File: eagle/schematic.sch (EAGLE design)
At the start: 4 parts, among them U1 SN74HC595N

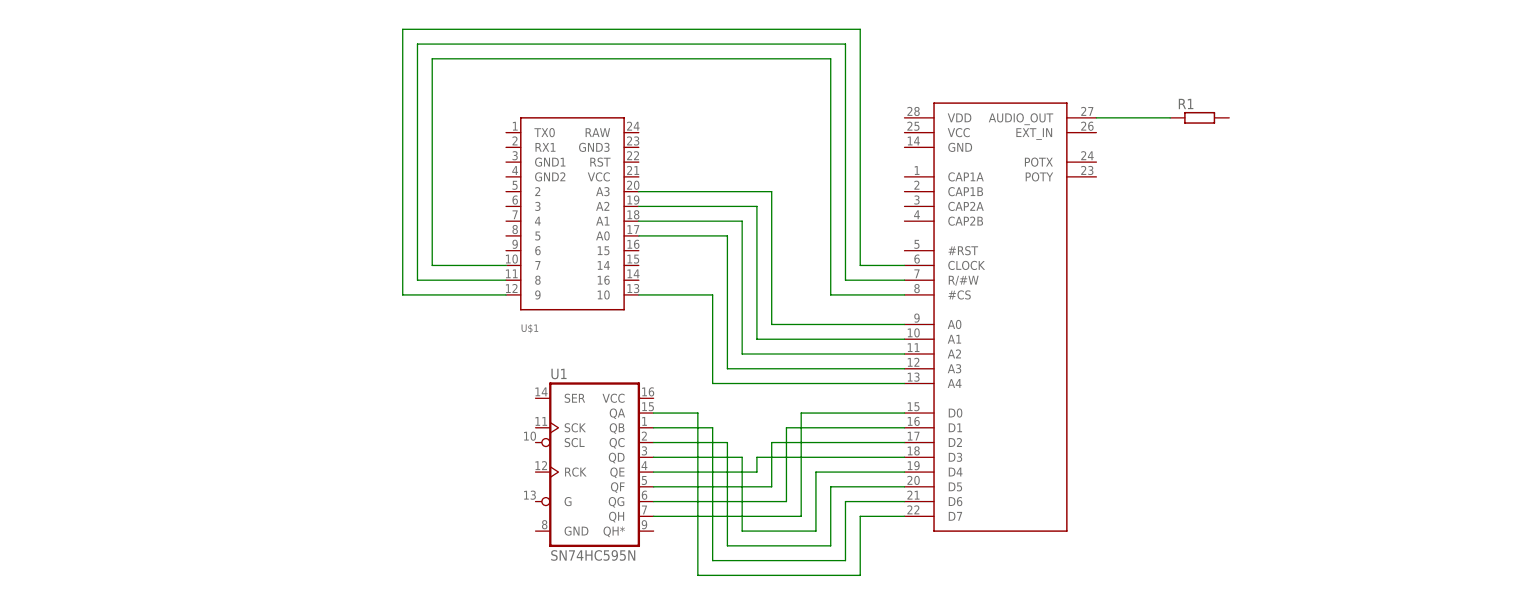
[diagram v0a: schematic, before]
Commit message: PCB update
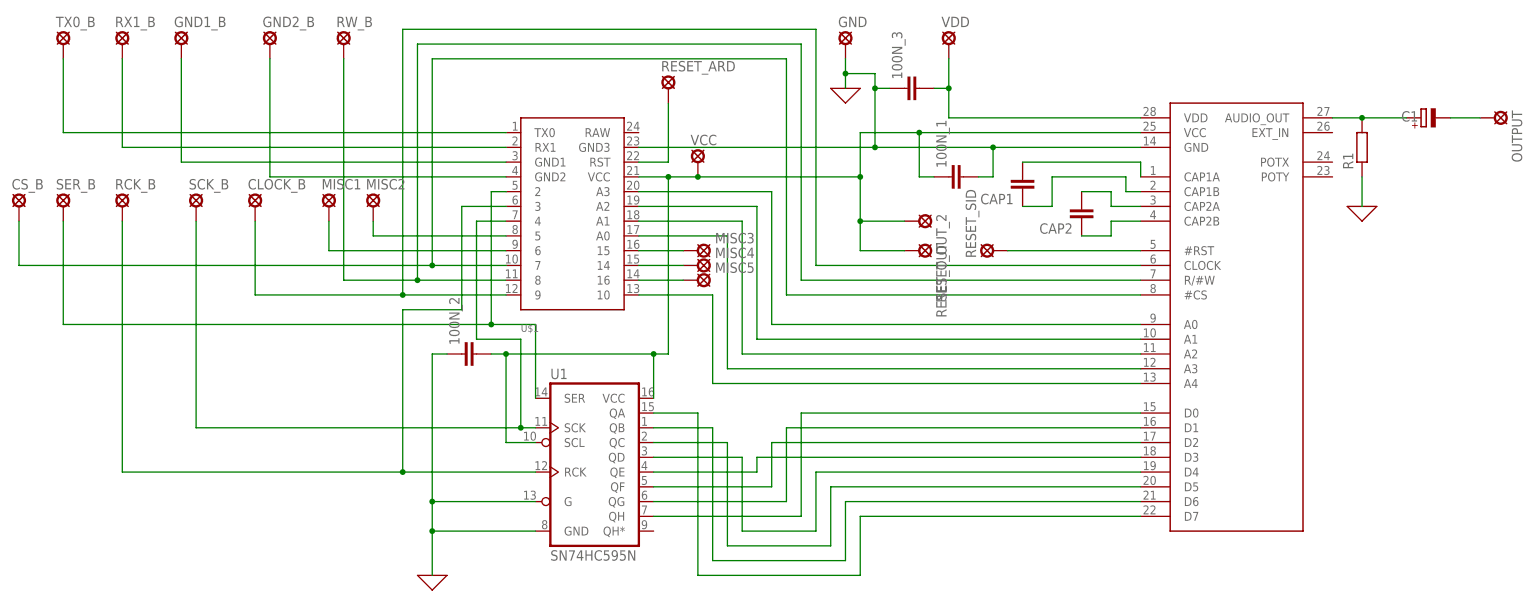
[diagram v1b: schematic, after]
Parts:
- added 100N_1: (no value), rcl:C-EU025-025X050
- added 100N_2, 100N_3, CAP1, CAP2: (no value), rcl:C-EU050-025X075
- added C1: (no value), rcl:CPOL-EUE2.5-5
- added CLOCK_B, CS_B, GND, GND1_B, GND2_B, MISC1, MISC2, MISC3, MISC4, MISC5, OUTPUT, RCK_B, RESET_ARD, RESET_OUT, RESET_OUT_2, RESET_SID, RW_B, RX1_B, SCK_B, SER_B, TX0_B, VCC, VDD: LSP11, solpad:LSP11
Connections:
- new net 0: 100N_1.2, 100N_2.1, 100N_3.1, GND.MP, R1.1, U$1.GND3, U$2.GND, U1.G, U1.GND
- new net N$18: 100N_3.2, U$2.VDD, VDD.MP
- new net N$19: 100N_1.1, 100N_2.2, RESET_OUT.MP, RESET_OUT_2.MP, U$1.VCC, U$2.VCC, U1.SCL, U1.VCC, VCC.MP
- new net N$20: CAP2.1, U$2.CAP2B
- new net N$21: RESET_SID.MP, U$2.#RST
- new net N$22: C1.-, OUTPUT.MP
- new net N$23: CAP2.2, U$2.CAP2A
- new net N$24: CAP1.2, U$2.CAP1A
- new net N$25: CAP1.1, U$2.CAP1B
- new net N$26: SER_B.MP, U$1.2, U1.SER
- new net N$27: SCK_B.MP, U$1.4, U1.SCK
- new net N$28: RCK_B.MP, U$1.3, U1.RCK
- new net N$29: MISC2.MP, U$1.5
- new net N$30: MISC1.MP, U$1.6
- new net N$31: RESET_ARD.MP, U$1.RST
- new net N$32: MISC3.MP, U$1.15
- new net N$33: MISC4.MP, U$1.14
- new net N$34: MISC5.MP, U$1.16
- new net N$35: TX0_B.MP, U$1.TX0
- new net N$36: RX1_B.MP, U$1.RX1
- new net N$37: GND1_B.MP, U$1.GND1
- new net N$38: GND2_B.MP, U$1.GND2
- net N$14: now also CS_B.MP
- net N$15: now also RW_B.MP
- net N$16: now also CLOCK_B.MP
- net N$17: now also C1.+, R1.2; no longer R1.1
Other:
- moved on the sheet: R1
